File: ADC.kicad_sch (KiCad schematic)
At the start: 14 parts, among them J301 Conn_01x04_Pin, U301 ADS122C04IPW

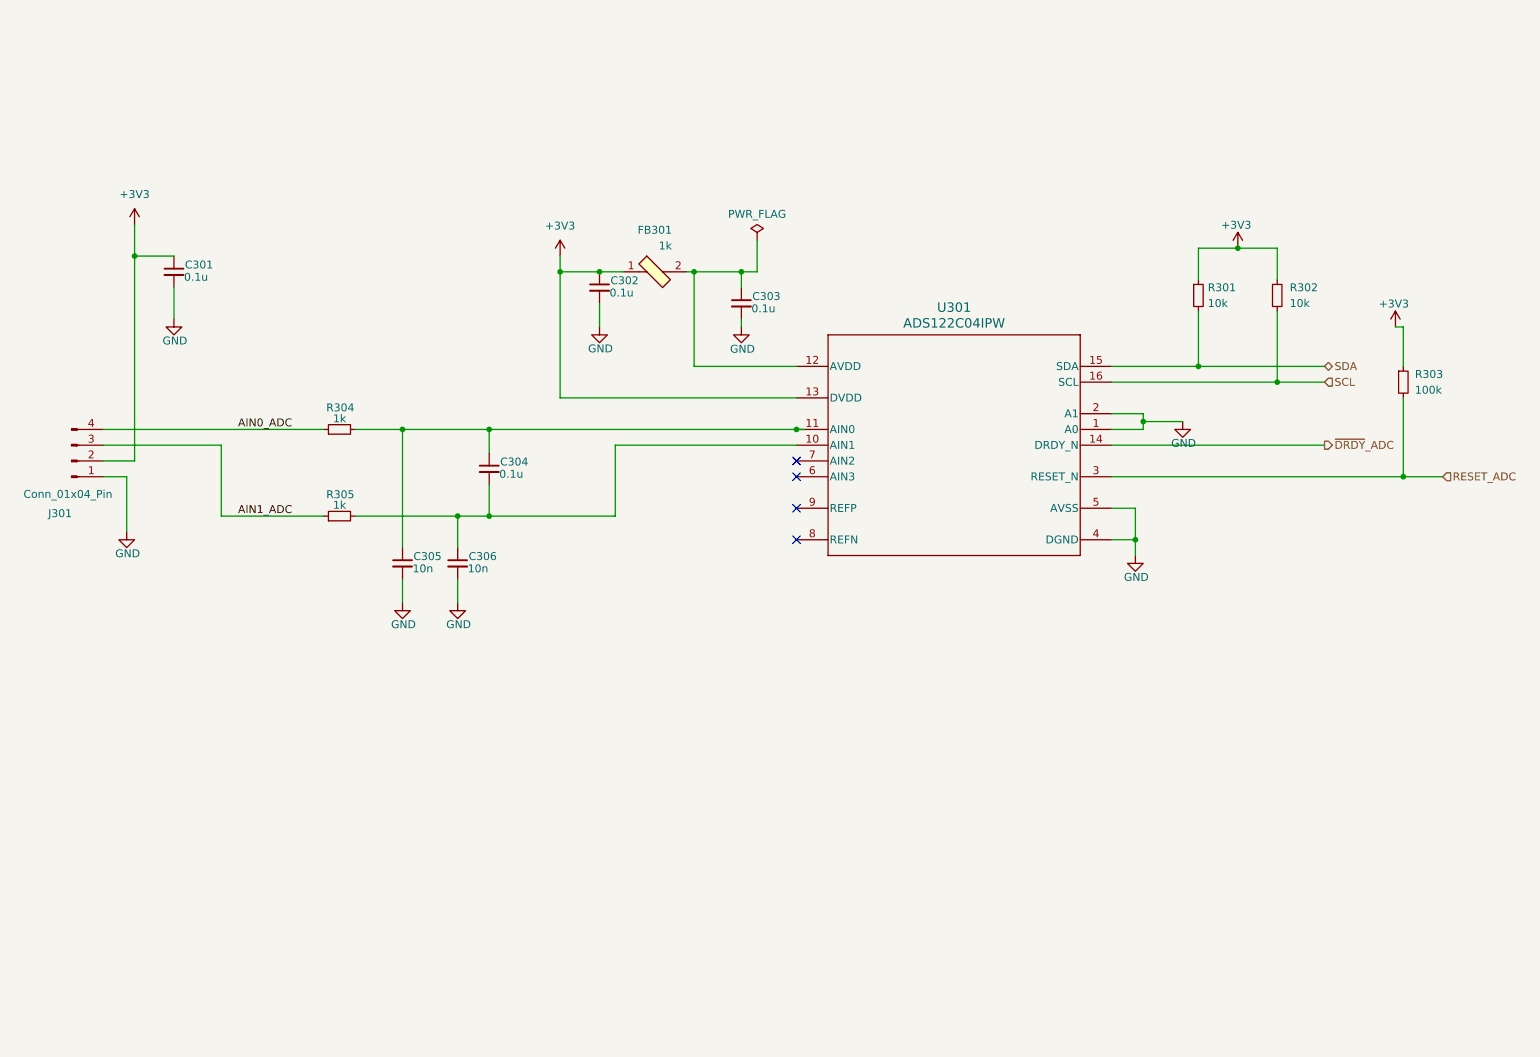
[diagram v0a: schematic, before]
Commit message: schematic pages are reviewed
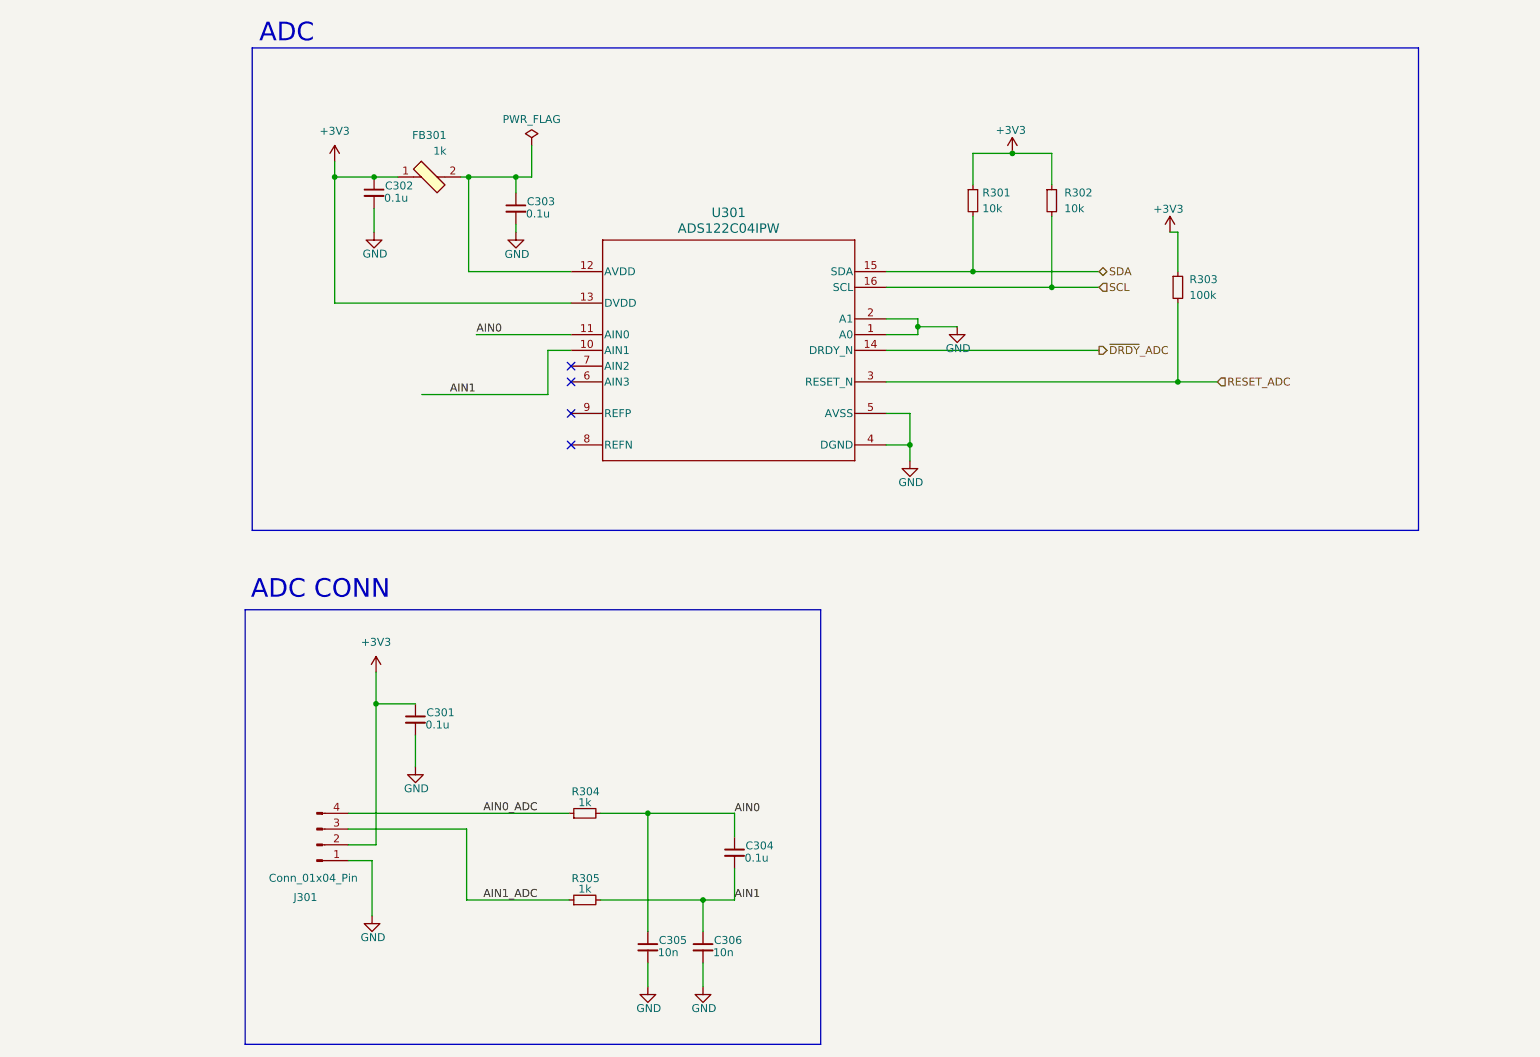
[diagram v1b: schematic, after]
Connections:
- net AIN1: now reaches C304.2, C306.1, R305.2, U301.10 (AIN1)
- net AIN0: now reaches C304.1, C305.1, R304.2, U301.11 (AIN0)
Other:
- note added: "ADC"
- note added: "ADC CONN"
- moved on the sheet: C301, C302, C303, C304, C305, C306, FB301, J301, R301, R302, R303, R304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
